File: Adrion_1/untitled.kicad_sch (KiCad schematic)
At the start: 2 parts, among them U2 NUCLEO-G474RE, U5 NUCLEO-G474RE

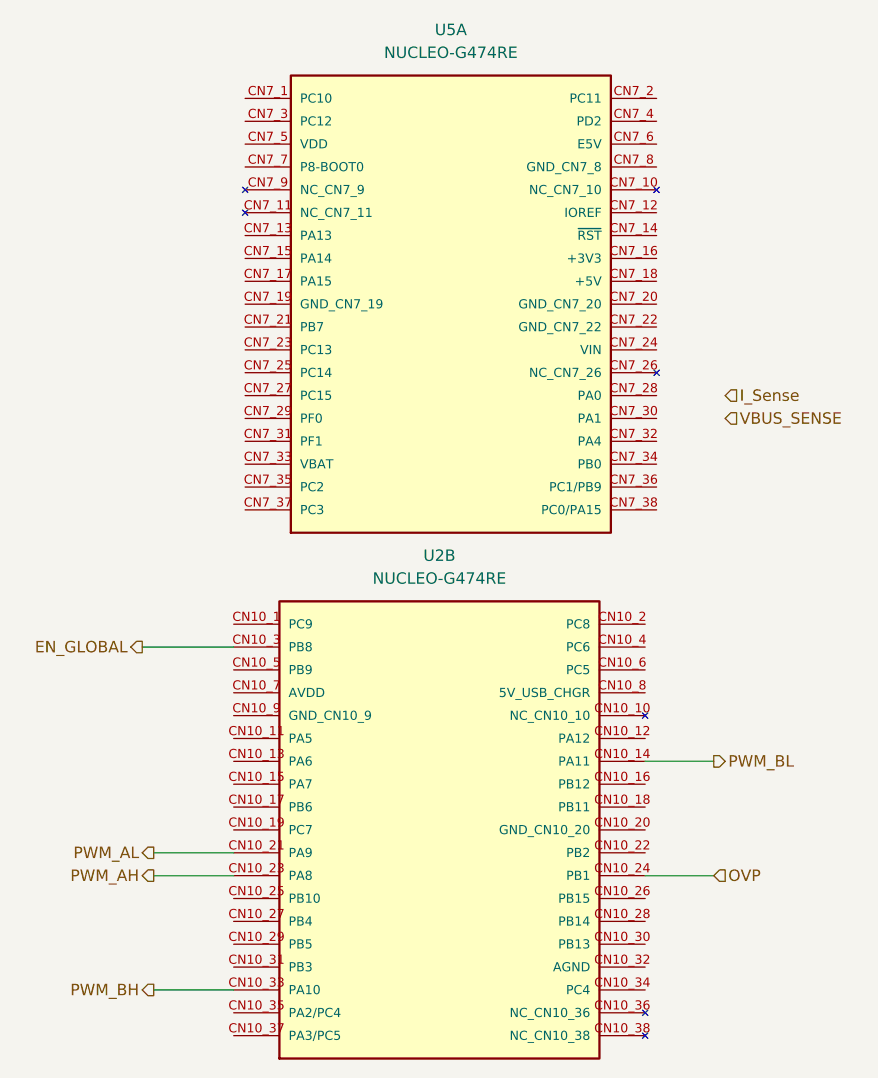
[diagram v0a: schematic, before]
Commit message: Correcciones
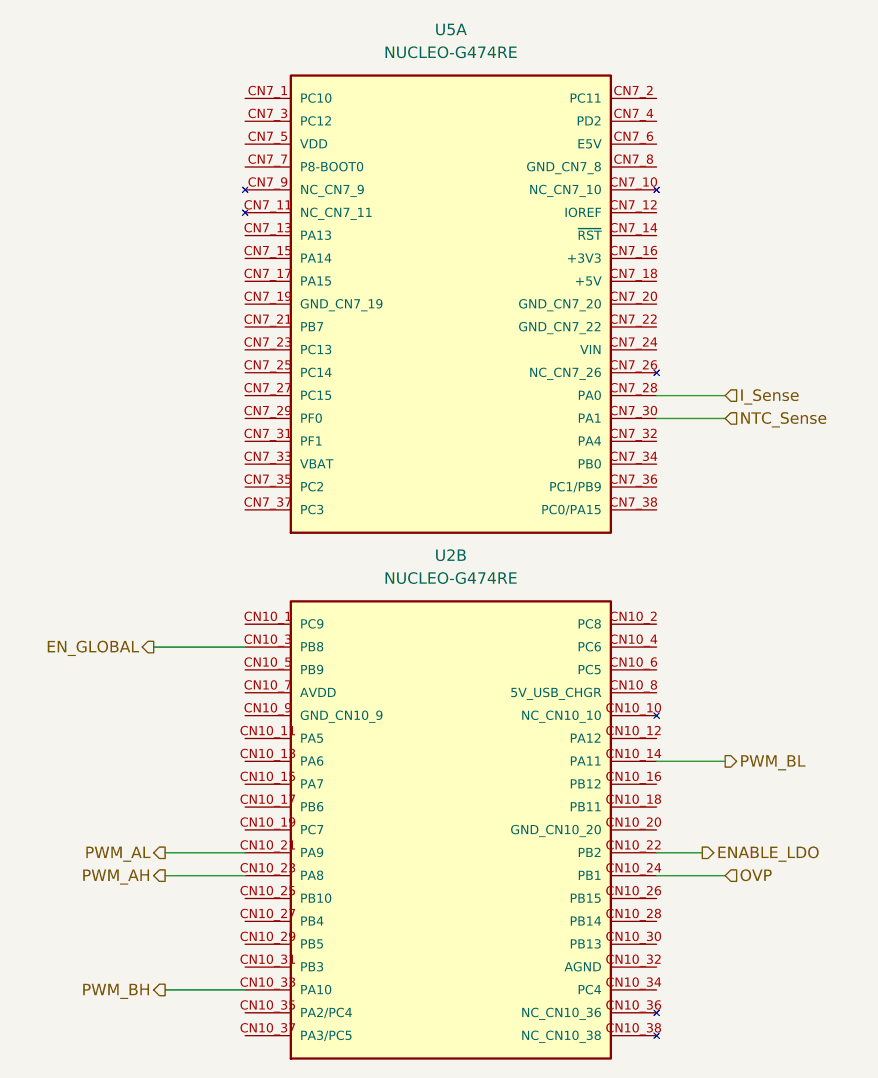
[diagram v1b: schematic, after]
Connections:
- net I_Sense: now also U5.CN7_28 (PA0)
- net ENABLE_LDO: now reaches U2.CN10_22 (PB2)
- net NTC_Sense: now reaches U5.CN7_30 (PA1)
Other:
- moved on the sheet: U2B
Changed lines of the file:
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@@
 	(wire
 		(pts
-			(xy 90.17 99.06) (xy 97.79 99.06)
-		)
-		(stroke
-			(width 0)
-			(type default)
-		)
-	)
-	(wire
-		(pts
-			(xy 90.17 111.76) (xy 97.79 111.76)
-		)
-		(stroke
-			(width 0)
-			(type default)
-		)
-	)
-	(wire
-		(pts
-			(xy 35.56 124.46) (xy 44.45 124.46)
-		)
-		(stroke
-			(width 0)
-			(type default)
-		)
-	)
-	(wire
-		(pts
-			(xy 35.56 111.76) (xy 44.45 111.76)
-		)
-		(stroke
-			(width 0)
-			(type default)
-		)
-	)
-	(wire
-		(pts
-			(xy 34.29 86.36) (xy 44.45 86.36)
-		)
-		(stroke
-			(width 0)
-			(type default)
-		)
-	)
-	(wire
-		(pts
-			(xy 35.56 109.22) (xy 44.45 109.22)
+			(xy 91.44 99.06) (xy 99.06 99.06)
+		)
+		(stroke
+			(width 0)
+			(type default)
+		)
+	)
+	(wire
+		(pts
+			(xy 91.44 111.76) (xy 99.06 111.76)
+		)
+		(stroke
+			(width 0)
+			(type default)
+		)
+	)
+	(wire
+		(pts
+			(xy 91.44 58.42) (xy 99.06 58.42)
+		)
+		(stroke
+			(width 0)
+			(type default)
+		)
+	)
+	(wire
+		(pts
+			(xy 36.83 124.46) (xy 45.72 124.46)
+		)
+		(stroke
+			(width 0)
+			(type default)
+		)
+	)
+	(wire
+		(pts
+			(xy 36.83 111.76) (xy 45.72 111.76)
+		)
+		(stroke
+			(width 0)
+			(type default)
+		)
+	)
+	(wire
+		(pts
+			(xy 35.56 86.36) (xy 45.72 86.36)
+		)
+		(stroke
+			(width 0)
+			(type default)
+		)
+	)
+	(wire
+		(pts
+			(xy 36.83 109.22) (xy 45.72 109.22)
+		)
+		(stroke
+			(width 0)
+			(type default)
+		)
+	)
+	(wire
+		(pts
+			(xy 91.44 109.22) (xy 96.52 109.22)
+		)
+		(stroke
+			(width 0)
+			(type default)
+		)
+	)
+	(wire
+		(pts
+			(xy 91.44 60.96) (xy 99.06 60.96)
 		)
 		(stroke
@@
 	(hierarchical_label "PWM_AH"
 		(shape output)
-		(at 35.56 111.76 180)
+		(at 36.83 111.76 180)
 		(effects
 			(font
@@
 	(hierarchical_label "PWM_BH"
 		(shape output)
-		(at 35.56 124.46 180)
+		(at 36.83 124.46 180)
 		(effects
 			(font
@@
 	(hierarchical_label "EN_GLOBAL"
 		(shape output)
-		(at 34.29 86.36 180)
+		(at 35.56 86.36 180)
 		(effects
 			(font
@@
 	(hierarchical_label "OVP"
 		(shape input)
-		(at 97.79 111.76 0)
-		(effects
-			(font
-				(size 1.27 1.27)
-			)
-			(justify left)
-		)
-	)
-	(hierarchical_label "VBUS_SENSE"
+		(at 99.06 111.76 0)
+		(effects
+			(font
+				(size 1.27 1.27)
+			)
+			(justify left)
+		)
+	)
+	(hierarchical_label "ENABLE_LDO"
+		(shape output)
+		(at 96.52 109.22 0)
+		(effects
+			(font
+				(size 1.27 1.27)
+			)
+			(justify left)
+		)
+	)
+	(hierarchical_label "PWM_BL"
+		(shape output)
+		(at 99.06 99.06 0)
+		(effects
+			(font
+				(size 1.27 1.27)
+			)
+			(justify left)
+		)
+	)
+	(hierarchical_label "NTC_Sense"
 		(shape input)
 		(at 99.06 60.96 0)
@@
 		)
 	)
-	(hierarchical_label "PWM_BL"
-		(shape output)
-		(at 97.79 99.06 0)
-		(effects
-			(font
-				(size 1.27 1.27)
-			)
-			(justify left)
-		)
-	)
 	(hierarchical_label "PWM_AL"
 		(shape output)
-		(at 35.56 109.22 180)
+		(at 36.83 109.22 180)
 		(effects
 			(font
@@
 	(symbol
 		(lib_id "NUCLEO-G474RE_3p:NUCLEO-G474RE")
-		(at 67.31 106.68 0)
+		(at 68.58 106.68 0)
 		(unit 2)
 		(exclude_from_sim no)
@@
 		(fields_autoplaced yes)
 		(property "Reference" "U2"
-			(at 67.31 76.2 0)
+			(at 68.58 76.2 0)
 			(effects
 				(font
@@
 		)
 		(property "Value" "NUCLEO-G474RE"
-			(at 67.31 78.74 0)
+			(at 68.58 78.74 0)
 			(effects
 				(font
@@
 		)
 		(property "Footprint" "NUCLEO-G474RE:MODULE_NUCLEO-G474RE"
-			(at 67.31 106.68 0)
+			(at 68.58 106.68 0)
 			(effects
 				(font
@@
 		)
 		(property "Datasheet" ""
-			(at 67.31 106.68 0)
+			(at 68.58 106.68 0)
 			(effects
 				(font
@@
 		)
 		(property "Description" ""
-			(at 67.31 106.68 0)
+			(at 68.58 106.68 0)
 			(effects
 				(font
@@
 		)
 		(property "MF" "STMicroelectronics"
-			(at 67.31 106.68 0)
+			(at 68.58 106.68 0)
 			(effects
 				(font
@@
 		)
 		(property "MAXIMUM_PACKAGE_HEIGHT" "20.7mm"
-			(at 67.31 106.68 0)
+			(at 68.58 106.68 0)
 			(effects
 				(font
@@
 		)
 		(property "Package" "None"
-			(at 67.31 106.68 0)
+			(at 68.58 106.68 0)
 			(effects
 				(font
@@
 		)
 		(property "Price" "None"
-			(at 67.31 106.68 0)
+			(at 68.58 106.68 0)
 			(effects
 				(font
@@
 		)
 		(property "Check_prices" "https://www.snapeda.com/parts/NUCLEO-G474RE/STMicroelectronics/view-part/?ref=eda"
-			(at 67.31 106.68 0)
+			(at 68.58 106.68 0)
 			(effects
 				(font
@@
 		)
 		(property "STANDARD" "Manufacturer Recommendations"
-			(at 67.31 106.68 0)
+			(at 68.58 106.68 0)
 			(effects
 				(font
@@
 		)
 		(property "PARTREV" "17"
-			(at 67.31 106.68 0)
+			(at 68.58 106.68 0)
 			(effects
 				(font
@@
 		)
 		(property "SnapEDA_Link" "https://www.snapeda.com/parts/NUCLEO-G474RE/STMicroelectronics/view-part/?ref=snap"
-			(at 67.31 106.68 0)
+			(at 68.58 106.68 0)
 			(effects
 				(font
@@
 		)
 		(property "MP" "NUCLEO-G474RE"
-			(at 67.31 106.68 0)
+			(at 68.58 106.68 0)
 			(effects
 				(font
@@
 		)
 		(property "Purchase-URL" "https://www.snapeda.com/api/url_track_click_mouser/?unipart_id=3662258&manufacturer=STMicroelectronics&part_name=NUCLEO-G474RE&search_term=None"
-			(at 67.31 106.68 0)
+			(at 68.58 106.68 0)
 			(effects
 				(font
@@
 		)
 		(property "Description_1" "STM32G474 Nucleo-64 STM32G4 ARM® Cortex®-M4 MCU 32-Bit Embedded Evaluation Board"
-			(at 67.31 106.68 0)
+			(at 68.58 106.68 0)
 			(effects
 				(font
@@
 		)
 		(property "Availability" "In Stock"
-			(at 67.31 106.68 0)
+			(at 68.58 106.68 0)
 			(effects
 				(font
@@
 		)
 		(property "MANUFACTURER" "STmicroelectronics"
-			(at 67.31 106.68 0)
-			(effects
-				(font
+			(at 68.58 106.68 0)
+			(effects
+				(font
